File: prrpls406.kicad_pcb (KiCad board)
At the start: 2 copper layers, 9 x 9 mm, 70 parts, among them U1001 ATtiny406-M

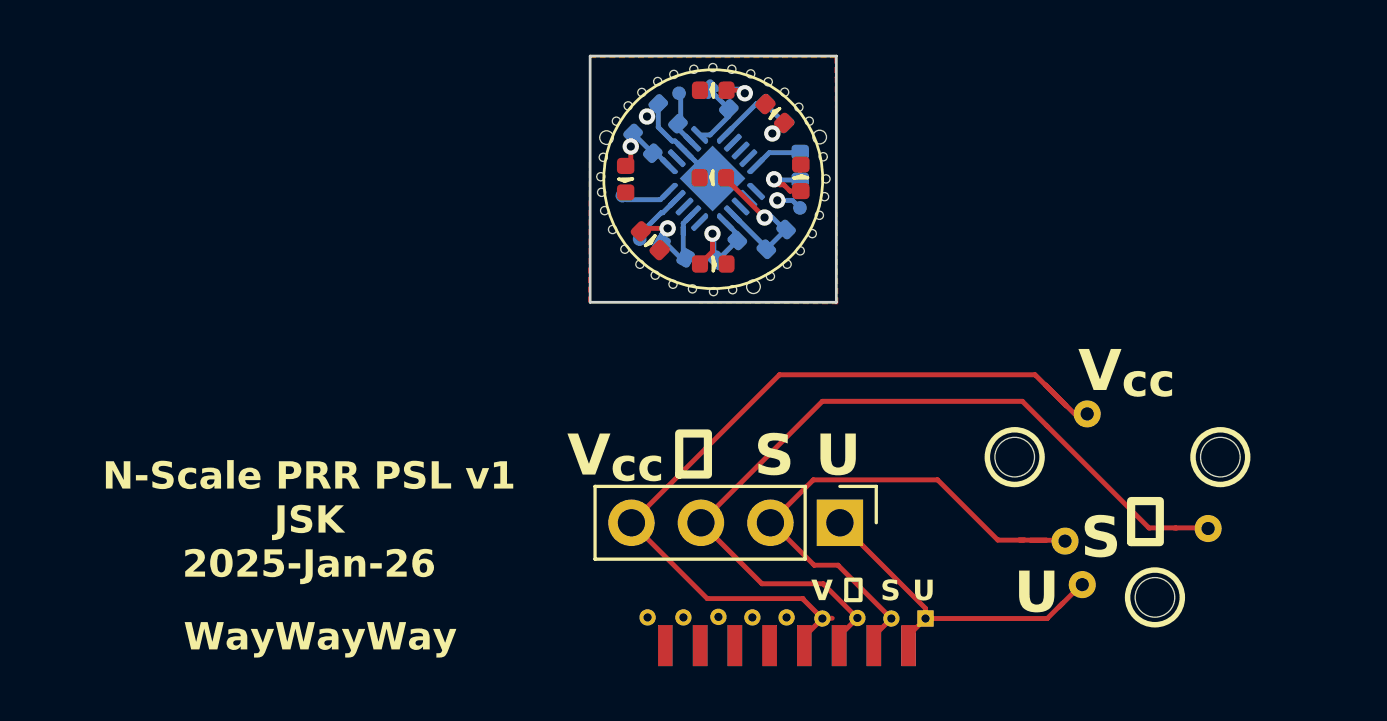
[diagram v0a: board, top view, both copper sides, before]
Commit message: made a new panel
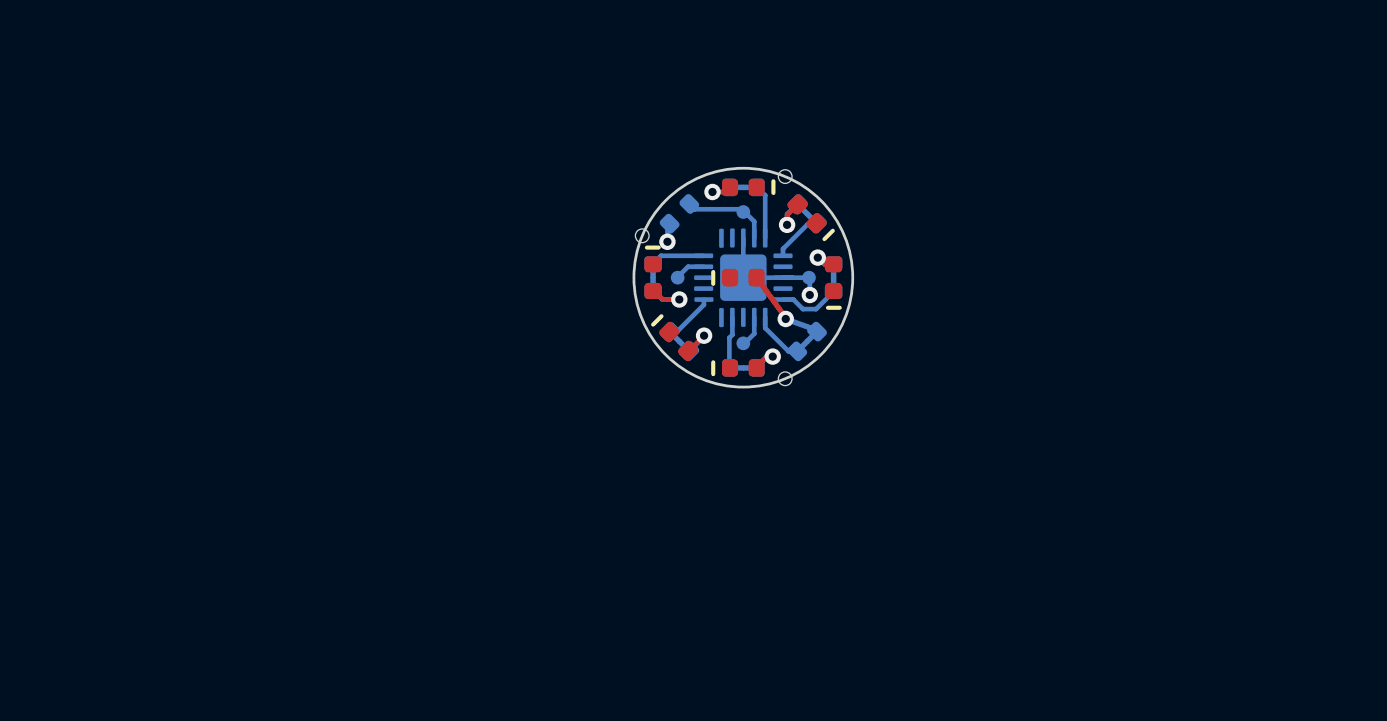
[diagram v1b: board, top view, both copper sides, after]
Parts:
- removed ?: , 
- removed H1001, H1003 (x3), H1004, H1005, H1006, H1008, H1009, H1010, H1012, H1013, H1014, H1015, H1017, H1018, H1019, H1020, H1021, H1022, H1023, H1024 (x3), H1026, H1027, H1028, H1030, H1031, H1032, H1033, H1035, H1036: MountingHole, JSK:0.3 npth
- removed H1007, H1016, H1029: MountingHole, JSK:0.5 npth
- removed the REF** at (135.0, 101.7)
- removed the REF** at (137.4, 96.6)
- removed the REF** at (129.9, 96.6)
- removed the REF** at (123.5, 99.0)
- removed the REF** at (132.4, 101.2)
- removed the REF** at (137.0, 99.2)
- removed the REF** at (131.8, 99.6)
- removed the REF** at (127.3, 103.6)
- removed the REF** at (132.6, 95.0)
- removed TP1001, TP1002, TP1003, TP1004: TestPoint, JSK:0.5mm-pogo-pad
- added H1: MountingHole, JSK:0.5 npth, F.Cu at (121.5, 86.3)
- added H2: MountingHole, JSK:0.5 npth, F.Cu at (116.3, 88.5)
- added H3: MountingHole, JSK:0.5 npth, F.Cu at (121.5, 93.7)
- added REF**: Tab, kikit:Tab, F.Cu at (117.7, 86.2)
- added REF**: Tab, kikit:Tab, F.Cu at (116.9, 93.2)
- added REF**: Tab, kikit:Tab, F.Cu at (124.4, 90.0)
- R1: renamed from R1007; footprint Resistor_SMD:R_0402_1005Metric -> JSK:Jumpered_R_0402_1005Metric
- R2: renamed from R1001; footprint Resistor_SMD:R_0402_1005Metric -> JSK:Jumpered_R_0402_1005Metric
- R3: renamed from R1002; footprint Resistor_SMD:R_0402_1005Metric -> JSK:Jumpered_R_0402_1005Metric
- R4: renamed from R1006; footprint Resistor_SMD:R_0402_1005Metric -> JSK:Jumpered_R_0402_1005Metric
- R5: renamed from R1004; footprint Resistor_SMD:R_0402_1005Metric -> JSK:Jumpered_R_0402_1005Metric
- R6: renamed from R1003; footprint Resistor_SMD:R_0402_1005Metric -> JSK:Jumpered_R_0402_1005Metric
- R7: renamed from R1005; footprint Resistor_SMD:R_0402_1005Metric -> JSK:Jumpered_R_0402_1005Metric
- U1: renamed from U1001; footprint Package_DFN_QFN:VQFN-20-1EP_3x3mm_P0.4mm_EP1.7x1.7mm -> JSK:extra_clearence_VQFN-20-1EP_3x3mm_P0.4mm_EP1.7x1.7mm
- moved R7 8.99 mm to (120.0, 93.3), turned to 0 degrees
- moved D1 8.14 mm to (123.3, 90.0), turned to 90 degrees
- moved D7 8.13 mm to (120.0, 93.3), turned to 0 degrees
- moved R1 7.76 mm to (123.3, 90.0), turned to 90 degrees
- moved TP3 6.98 mm to (120.0, 92.4), turned to 0 degrees
- moved TP2 4.94 mm to (120.0, 87.6), turned to 0 degrees
- moved R4 3.90 mm to (122.3, 92.3)
- moved D2 3.85 mm to (122.3, 87.7), turned to 135 degrees
- moved R2 3.85 mm to (122.3, 87.7), turned to 135 degrees
- moved D6 3.83 mm to (117.6, 92.3), turned to -45 degrees
- moved D4 3.82 mm to (120.0, 90.0)
- moved U1 3.80 mm to (120.0, 90.0), turned to -90 degrees
- moved C1 3.68 mm to (117.7, 87.7), turned to -135 degrees
- moved R6 3.32 mm to (117.7, 92.3), turned to -45 degrees
- moved R5 2.90 mm to (116.7, 90.0), turned to -90 degrees
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- renumbered C1001 to C1, D1001 to D1, D1002 to D2, D1003 to D3, D1007 to D4, D1004 to D5, D1005 to D6, D1006 to D7, TP1002 to TP1, TP1004 to TP2, TP1003 to TP3, TP1001 to TP4
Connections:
- R1 pad 1: Net-(U1001-PA4) -> Net-(U1-PB4)
- R3 pad 1: Net-(U1001-PB4) -> Net-(U1-PA4)
- R4 pad 1: Net-(U1001-PB0) -> Net-(U1-PB3)
- R5 pad 1: Net-(U1001-PC0) -> Net-(U1-PA1)
- R6 pad 1: Net-(U1001-PC2) -> Net-(U1-PC1)
- R7 pad 1: Net-(U1001-PA2) -> Net-(U1-PB0)
- U1 pad 1: Net-(U1001-PA2) -> unconnected-(U1-PA2-Pad1)
- U1 pad 10: Net-(U1001-PB4) -> Net-(U1-PB4)
- U1 pad 11: unconnected-(U1001-PB3-Pad11) -> Net-(U1-PB3)
- U1 pad 12: unconnected-(U1001-PB2-Pad12) -> /Serial
- U1 pad 14: Net-(U1001-PB0) -> Net-(U1-PB0)
- U1 pad 15: Net-(U1001-PC0) -> unconnected-(U1-PC0-Pad15)
- U1 pad 16: unconnected-(U1001-PC1-Pad16) -> Net-(U1-PC1)
- U1 pad 17: Net-(U1001-PC2) -> unconnected-(U1-PC2-Pad17)
- U1 pad 20: /Serial -> Net-(U1-PA1)
- U1 pad 5: Net-(U1001-PA4) -> Net-(U1-PA4)
- U1 pad 8: unconnected-(U1001-PA7-Pad8) -> GND
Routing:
- net (no net): track 93.7 -> 0.00 mm
- net Net-(D1-A): track 10.2 -> 1.35 mm
- net Net-(U1-PB4): track 0.00 -> 2.25 mm
- net Net-(U1001-PC2): track 2.00 -> 0.00 mm
- net Net-(U1-PA4): track 0.00 -> 1.95 mm
- net Net-(U1-PA1): track 0.00 -> 1.95 mm
- net Net-(U1-PB3): track 0.00 -> 1.92 mm
- net Net-(U1-PB0): track 0.00 -> 1.85 mm
- net Net-(U1001-PB4): track 1.82 -> 0.00 mm
- net Net-(U1-PC1): track 0.00 -> 1.80 mm
- net Net-(U1001-PB0): track 1.78 -> 0.00 mm
- net Net-(U1001-PA4): track 1.61 -> 0.00 mm
- net Net-(U1001-PA2): track 1.11 -> 0.00 mm
- net +5V: track 2.09 -> 3.19 mm
- net /UPDI: track 2.07 -> 1.14 mm
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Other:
- board size 9 x 9 mm -> 8 x 8 mm
- board text removed: "N-Scale PRR PSL v1 JSK 2025-Jan-26"
- board text removed: "S"
- board text removed: "U"
- board text removed: "V"
- board text removed: "V_{cc}"
- board text removed: "WayWayWay"
- board text removed: "⏚"
